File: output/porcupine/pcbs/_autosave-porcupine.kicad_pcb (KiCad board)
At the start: 2 copper layers, 140.5 x 103.1 mm, 38 parts, among them J1 Jumper, J2 Jumper

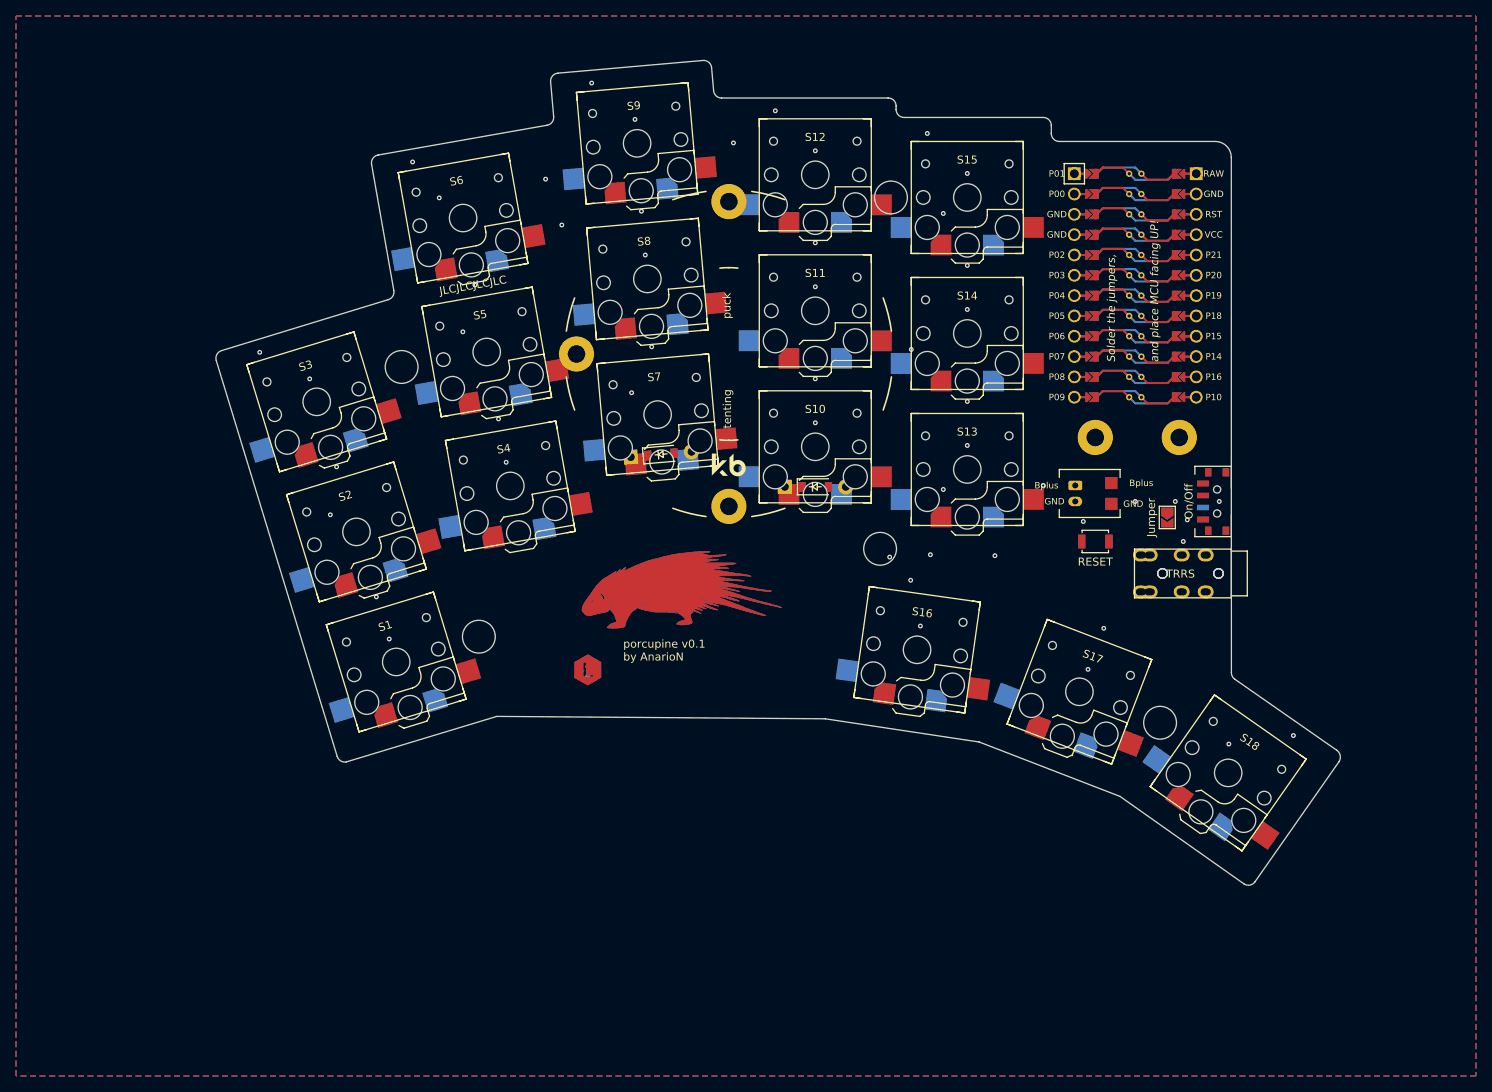
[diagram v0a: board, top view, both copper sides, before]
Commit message: Beschreibung deiner Änderungen
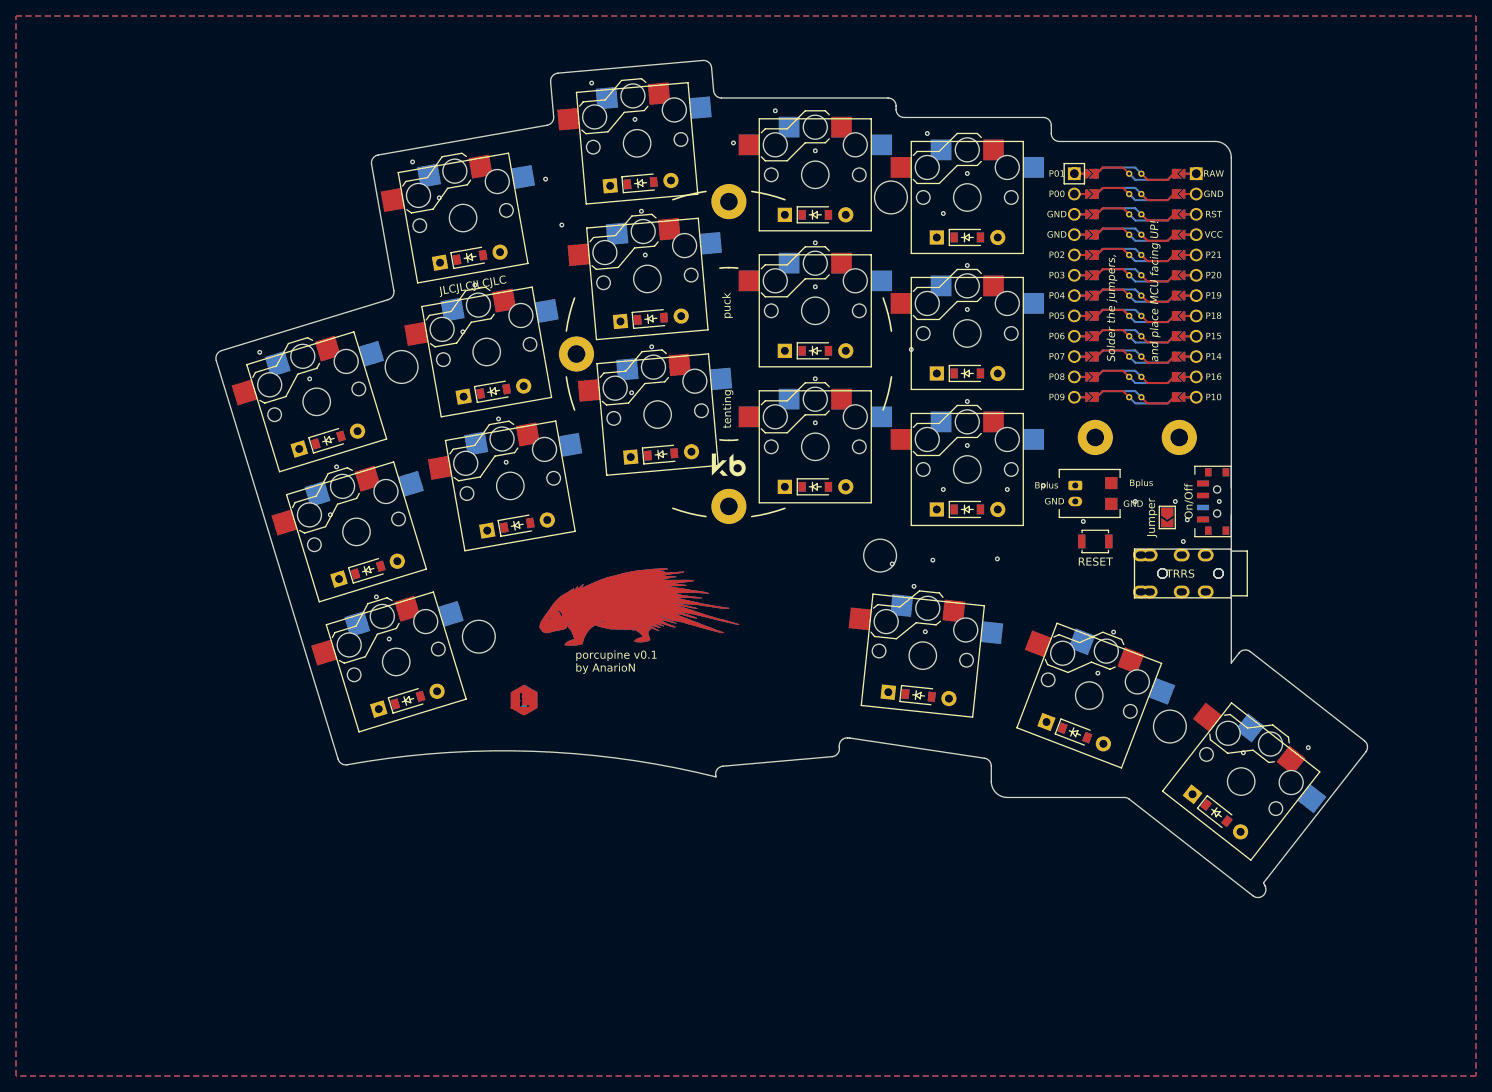
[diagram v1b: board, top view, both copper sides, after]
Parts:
- added D1: D_SOD-123, Diode_SMD:SOD-123, F.Cu at (176.5, 155.5)
- added D11: D_SOD-123, Diode_SMD:SOD-123, F.Cu at (227.4, 111.9)
- added D12: D_SOD-123, Diode_SMD:SOD-123, F.Cu at (227.4, 94.9)
- added D13: D_SOD-123, Diode_SMD:SOD-123, F.Cu at (246.4, 131.7)
- added D14: D_SOD-123, Diode_SMD:SOD-123, F.Cu at (246.4, 114.7)
- added D15: D_SOD-123, Diode_SMD:SOD-123, F.Cu at (246.4, 97.7)
- added D16: D_SOD-123, Diode_SMD:SOD-123, F.Cu at (240.3, 154.9)
- added D17: D_SOD-123, Diode_SMD:SOD-123, F.Cu at (259.9, 159.6)
- added D18: D_SOD-123, Diode_SMD:SOD-123, F.Cu at (277.6, 169.6)
- added D2: D_SOD-123, Diode_SMD:SOD-123, F.Cu at (171.5, 139.3)
- added D3: D_SOD-123, Diode_SMD:SOD-123, F.Cu at (166.6, 123.0)
- added D4: D_SOD-123, Diode_SMD:SOD-123, F.Cu at (190.2, 133.7)
- added D5: D_SOD-123, Diode_SMD:SOD-123, F.Cu at (187.2, 116.9)
- added D6: D_SOD-123, Diode_SMD:SOD-123, F.Cu at (184.3, 100.2)
- added D8: D_SOD-123, Diode_SMD:SOD-123, F.Cu at (206.9, 107.8)
- added D9: D_SOD-123, Diode_SMD:SOD-123, F.Cu at (205.6, 90.9)
- S1, S10, S11, S12, S13, S14, S15, S16, S17, S18, S2, S3, S4, S5, S6, S7, S8, S9: footprint Keyboards:Kailh_socket_PG1350_reversible_cropped_pads -> PG1350
- moved Side_B 8.80 mm to (189.6, 158.4)
- moved Side_F 8.80 mm to (189.6, 154.5)
- moved LOGO_B 5.71 mm to (205.4, 143.9)
- moved LOGO_F 5.71 mm to (205.4, 143.9)
- moved S18 1.95 mm to (280.7, 165.7), turned to -38 degrees
- moved S17 1.32 mm to (261.7, 154.9)
- moved S16 1.02 mm to (240.9, 150.0), turned to -6 degrees
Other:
- board size 140.5 x 103.1 mm -> 143.9 x 104.6 mm
